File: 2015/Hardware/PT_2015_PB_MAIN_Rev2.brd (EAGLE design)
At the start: 137.2 x 166.4 mm, 135 parts, among them Q1 Q_ACS711LC, Q11 Q_IRFS7437PbF, Q12 2N7002, Q14 Q_IRFS7437PbF, Q16 Q_IRFS7437PbF, Q18 Q_FDT86102LZ, Q20 Q_IRFS7437PbF, Q4 Q_ACS711LC, Q5 Q_ACS711LC, Q6 Q_IRFS7437PbF, Q7 Q_IRFS7437PbF, Q9 Q_IRFS7437PbF

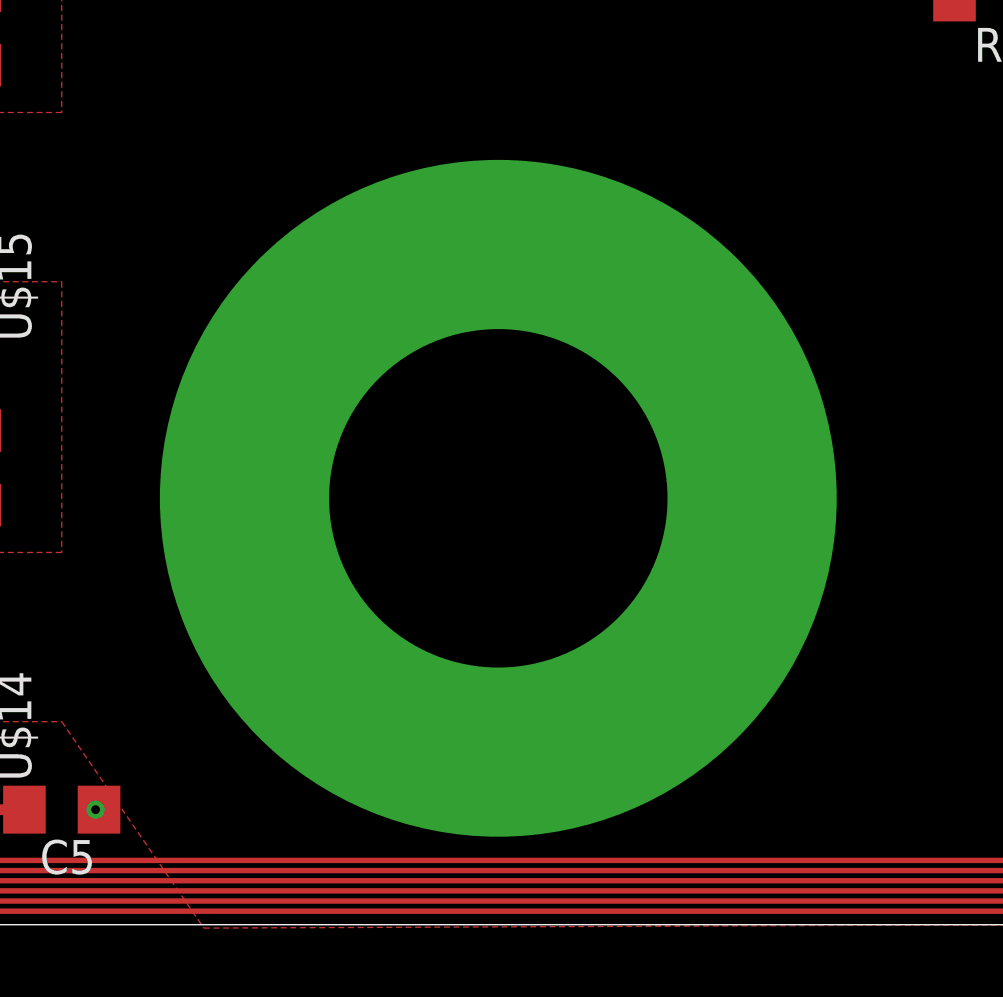
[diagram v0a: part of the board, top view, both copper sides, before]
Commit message: Oh yeah BTW this is basically done
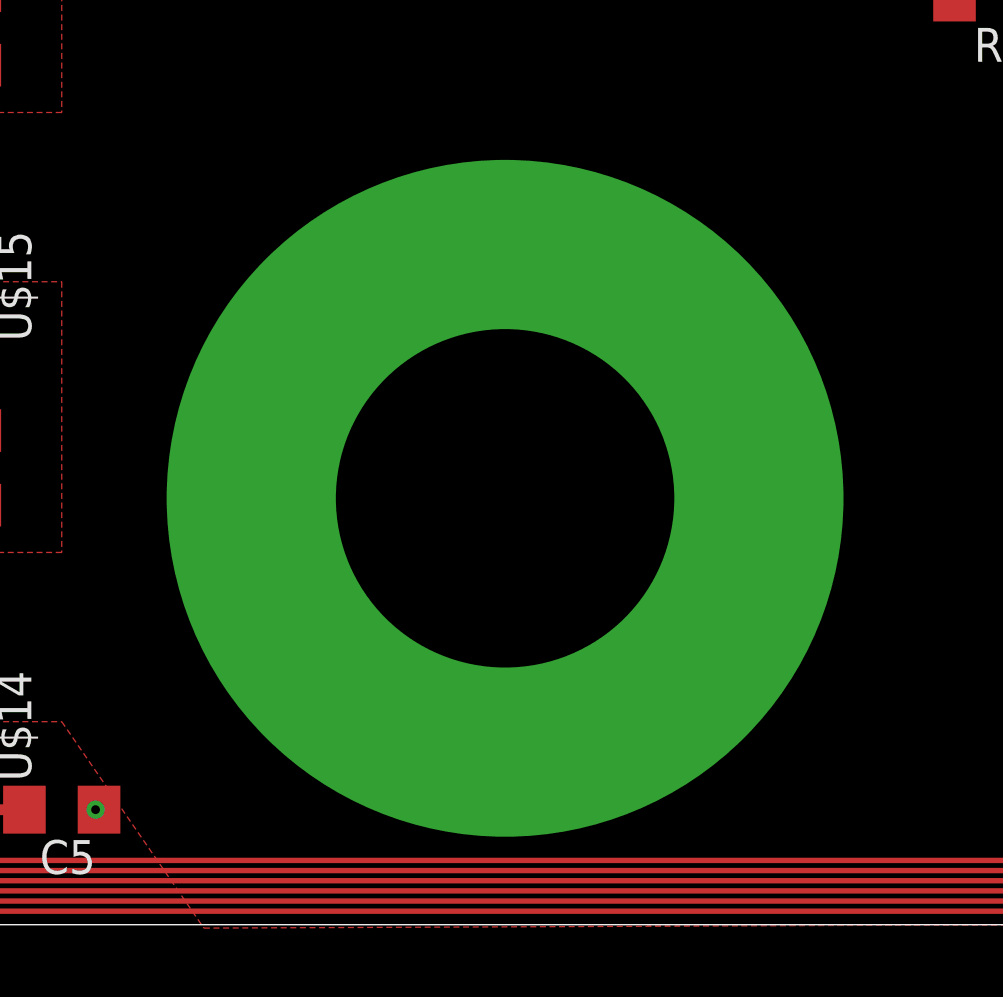
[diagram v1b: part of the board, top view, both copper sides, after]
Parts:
- moved BATT-POS 0.25 mm to (62.4, 13.5)
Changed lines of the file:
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@@
 <element name="C10" library="resistor" package="C1206" value="" x="81.153" y="52.197" rot="R180"/>
 <element name="C14" library="resistor" package="C1206" value="2.2µF" x="81.28" y="68.58" rot="R270"/>
-<element name="BATT-POS" library="MRDT-2015-PowerBoard" package="LARGE_TERMINAL_HOLE" value="TERMINAL_HOLE" x="62.103" y="13.462"/>
+<element name="BATT-POS" library="MRDT-2015-PowerBoard" package="LARGE_TERMINAL_HOLE" value="TERMINAL_HOLE" x="62.357" y="13.462"/>
 <element name="BATT-NEG" library="MRDT-2015-PowerBoard" package="LARGE_TERMINAL_HOLE" value="TERMINAL_HOLE" x="93.98" y="13.462"/>
 <element name="Q6" library="MRDT-2015-PowerBoard" package="D2PACK" value="Q_IRFS7437PbF" x="29.21" y="7.62" rot="R270"/>
